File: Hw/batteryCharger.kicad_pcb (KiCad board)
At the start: 2 copper layers, 12.2 x 17.4 mm, 15 parts, among them J1 Vcc, J2 GND, J3 BAT, J4 GND, U1 MCP73831-2-OT

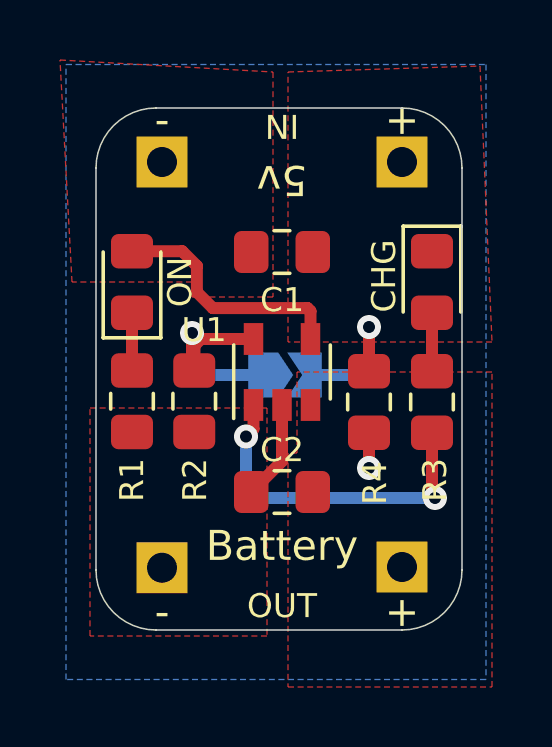
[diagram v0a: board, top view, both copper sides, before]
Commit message: Update_kicad_6
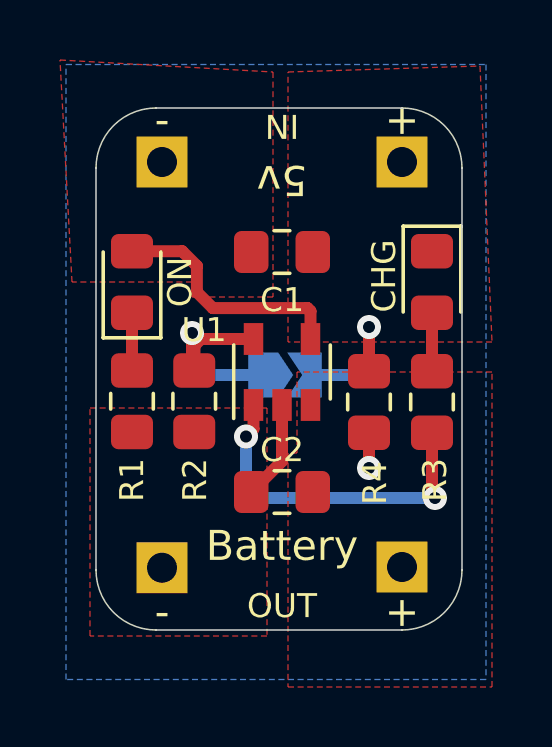
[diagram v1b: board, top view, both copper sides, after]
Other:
- net class Default removed
